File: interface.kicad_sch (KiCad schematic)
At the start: 8 parts

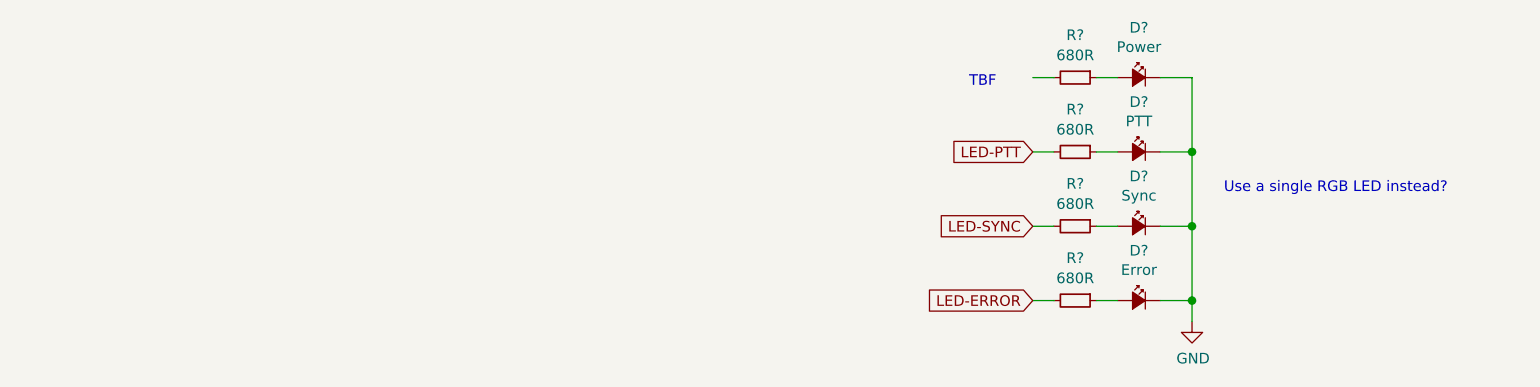
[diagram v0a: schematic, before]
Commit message: Add files via upload
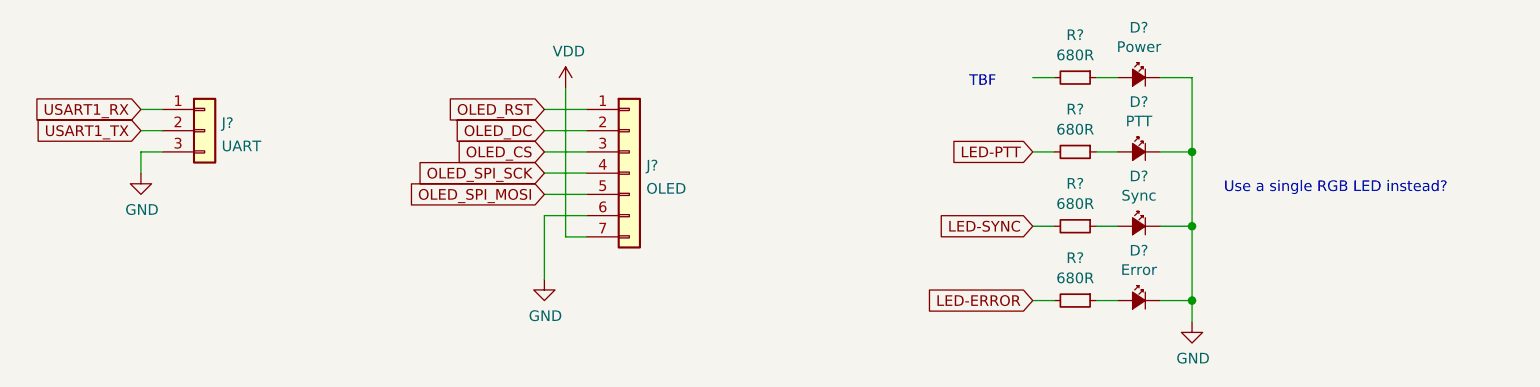
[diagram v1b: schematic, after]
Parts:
- added J?: OLED, Connector_PinHeader_2.54mm:PinHeader_1x07_P2.54mm_Vertical, symbol Connector_Generic:Conn_01x07
- added J?: UART, Connector_PinHeader_2.54mm:PinHeader_1x03_P2.54mm_Vertical, symbol Connector_Generic:Conn_01x03
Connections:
- net GND: now also J?.3 (Pin_3), J?.6 (Pin_6)
- new net OLED_CS: J?.3 (Pin_3)
- new net OLED_DC: J?.2 (Pin_2)
- new net OLED_RST: J?.1 (Pin_1)
- new net OLED_SPI_MOSI: J?.5 (Pin_5)
- new net OLED_SPI_SCK: J?.4 (Pin_4)
- new net USART1_RX: J?.1 (Pin_1)
- new net USART1_TX: J?.2 (Pin_2)
- new net VDD: J?.7 (Pin_7)
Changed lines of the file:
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@@
+    (stroke (width 0) (type solid) (color 0 0 0 0))
+  )
+  (wire (pts (xy 130.81 93.98) (xy 135.89 93.98))
     (stroke (width 0) (type solid) (color 0 0 0 0))
   )
@@
     (stroke (width 0) (type solid) (color 0 0 0 0))
   )
+  (wire (pts (xy 82.55 96.52) (xy 85.09 96.52))
+    (stroke (width 0) (type solid) (color 0 0 0 0))
+  )
   (wire (pts (xy 204.47 90.17) (xy 208.28 90.17))
     (stroke (width 0) (type solid) (color 0 0 0 0))
@@
     (stroke (width 0) (type solid) (color 0 0 0 0))
   )
+  (wire (pts (xy 135.89 106.68) (xy 130.81 106.68))
+    (stroke (width 0) (type solid) (color 0 0 0 0))
+  )
   (wire (pts (xy 208.28 116.84) (xy 208.28 119.38))
     (stroke (width 0) (type solid) (color 0 0 0 0))
@@
     (stroke (width 0) (type solid) (color 0 0 0 0))
   )
+  (wire (pts (xy 135.89 109.22) (xy 133.35 109.22))
+    (stroke (width 0) (type solid) (color 0 0 0 0))
+  )
   (wire (pts (xy 208.28 107.95) (xy 208.28 116.84))
     (stroke (width 0) (type solid) (color 0 0 0 0))
   )
+  (wire (pts (xy 133.35 109.22) (xy 133.35 91.44))
+    (stroke (width 0) (type solid) (color 0 0 0 0))
+  )
+  (wire (pts (xy 82.55 93.98) (xy 85.09 93.98))
+    (stroke (width 0) (type solid) (color 0 0 0 0))
+  )
   (wire (pts (xy 208.28 90.17) (xy 208.28 99.06))
     (stroke (width 0) (type solid) (color 0 0 0 0))
   )
+  (wire (pts (xy 130.81 101.6) (xy 135.89 101.6))
+    (stroke (width 0) (type solid) (color 0 0 0 0))
+  )
   (wire (pts (xy 196.85 99.06) (xy 199.39 99.06))
     (stroke (width 0) (type solid) (color 0 0 0 0))
   )
+  (wire (pts (xy 130.81 96.52) (xy 135.89 96.52))
+    (stroke (width 0) (type solid) (color 0 0 0 0))
+  )
+  (wire (pts (xy 130.81 106.68) (xy 130.81 114.3))
+    (stroke (width 0) (type solid) (color 0 0 0 0))
+  )
+  (wire (pts (xy 85.09 99.06) (xy 82.55 99.06))
+    (stroke (width 0) (type solid) (color 0 0 0 0))
+  )
   (wire (pts (xy 191.77 90.17) (xy 189.23 90.17))
     (stroke (width 0) (type solid) (color 0 0 0 0))
   )
   (wire (pts (xy 204.47 107.95) (xy 208.28 107.95))
+    (stroke (width 0) (type solid) (color 0 0 0 0))
+  )
+  (wire (pts (xy 82.55 99.06) (xy 82.55 101.6))
+    (stroke (width 0) (type solid) (color 0 0 0 0))
+  )
+  (wire (pts (xy 130.81 99.06) (xy 135.89 99.06))
+    (stroke (width 0) (type solid) (color 0 0 0 0))
+  )
+  (wire (pts (xy 130.81 104.14) (xy 135.89 104.14))
     (stroke (width 0) (type solid) (color 0 0 0 0))
   )
@@
     (effects (font (size 1.27 1.27)) (justify left bottom))
   )
+  (global_label "OLED_SPI_SCK" (shape input) (at 130.81 101.6 180) (fields_autoplaced)
+    (effects (font (size 1.27 1.27)) (justify right))
+    (property "Intersheet References" "${INTERSHEET_REFS}" (id 0) (at 114.9899 101.5206 0)
+      (effects (font (size 1.27 1.27)) (justify right) hide)
+    )
+  )
+  (global_label "OLED_DC" (shape input) (at 130.81 96.52 180) (fields_autoplaced)
+    (effects (font (size 1.27 1.27)) (justify right))
+    (property "Intersheet References" "${INTERSHEET_REFS}" (id 0) (at 120.2514 96.4406 0)
+      (effects (font (size 1.27 1.27)) (justify right) hide)
+    )
+  )
   (global_label "LED-PTT" (shape input) (at 189.23 99.06 180) (fields_autoplaced)
     (effects (font (size 1.27 1.27)) (justify right))
@@
     )
   )
+  (global_label "OLED_SPI_MOSI" (shape input) (at 130.81 104.14 180) (fields_autoplaced)
+    (effects (font (size 1.27 1.27)) (justify right))
+    (property "Intersheet References" "${INTERSHEET_REFS}" (id 0) (at 114.1433 104.0606 0)
+      (effects (font (size 1.27 1.27)) (justify right) hide)
+    )
+  )
   (global_label "LED-SYNC" (shape input) (at 189.23 107.95 180) (fields_autoplaced)
     (effects (font (size 1.27 1.27)) (justify right))
@@
     )
   )
+  (global_label "USART1_RX" (shape input) (at 82.55 93.98 180) (fields_autoplaced)
+    (effects (font (size 1.27 1.27)) (justify right))
+    (property "Intersheet References" "${INTERSHEET_REFS}" (id 0) (at 69.7537 94.0594 0)
+      (effects (font (size 1.27 1.27)) (justify right) hide)
+    )
+  )
+  (global_label "USART1_TX" (shape input) (at 82.55 96.52 180) (fields_autoplaced)
+    (effects (font (size 1.27 1.27)) (justify right))
+    (property "Intersheet References" "${INTERSHEET_REFS}" (id 0) (at 70.0561 96.5994 0)
+      (effects (font (size 1.27 1.27)) (justify right) hide)
+    )
+  )
+  (global_label "OLED_CS" (shape input) (at 130.81 99.06 180) (fields_autoplaced)
+    (effects (font (size 1.27 1.27)) (justify right))
+    (property "Intersheet References" "${INTERSHEET_REFS}" (id 0) (at 120.3118 98.9806 0)
+      (effects (font (size 1.27 1.27)) (justify right) hide)
+    )
+  )
   (global_label "LED-ERROR" (shape input) (at 189.23 116.84 180) (fields_autoplaced)
     (effects (font (size 1.27 1.27)) (justify right))
     (property "Intersheet References" "${INTERSHEET_REFS}" (id 0) (at -72.39 -38.1 0)
       (effects (font (size 1.27 1.27)) hide)
+    )
+  )
+  (global_label "OLED_RST" (shape input) (at 130.81 93.98 180) (fields_autoplaced)
+    (effects (font (size 1.27 1.27)) (justify right))
+    (property "Intersheet References" "${INTERSHEET_REFS}" (id 0) (at 119.3442 93.9006 0)
+      (effects (font (size 1.27 1.27)) (justify right) hide)
     )
   )
@@
     (pin "C")
   )
+  (symbol (lib_id "power:GND") (at 82.55 101.6 0) (unit 1)
+    (in_bom yes) (on_board yes)
+    (property "Reference" "#PWR?" (id 0) (at 82.55 107.95 0)
+      (effects (font (size 1.27 1.27)) hide)
+    )
+    (property "Value" "GND" (id 1) (at 82.677 105.9942 0))
+    (property "Footprint" "" (id 2) (at 82.55 101.6 0)
+      (effects (font (size 1.27 1.27)) hide)
+    )
+    (property "Datasheet" "" (id 3) (at 82.55 101.6 0)
+      (effects (font (size 1.27 1.27)) hide)
+    )
+    (pin "1")
+  )
+  (symbol (lib_id "power:VDD") (at 133.35 91.44 0) (unit 1)
+    (in_bom yes) (on_board yes)
+    (property "Reference" "#PWR?" (id 0) (at 133.35 95.25 0)
+      (effects (font (size 1.27 1.27)) hide)
+    )
+    (property "Value" "VDD" (id 1) (at 133.731 87.0458 0))
+    (property "Footprint" "" (id 2) (at 133.35 91.44 0)
+      (effects (font (size 1.27 1.27)) hide)
+    )
+    (property "Datasheet" "" (id 3) (at 133.35 91.44 0)
+      (effects (font (size 1.27 1.27)) hide)
+    )
+    (pin "1")
+  )
+  (symbol (lib_id "Connector_Generic:Conn_01x07") (at 140.97 101.6 0) (unit 1)
+    (in_bom yes) (on_board yes) (fields_autoplaced)
+    (property "Reference" "J?" (id 0) (at 143.0021 100.6915 0)
+      (effects (font (size 1.27 1.27)) (justify left))
+    )
+    (property "Value" "OLED" (id 1) (at 143.0021 103.4666 0)
+      (effects (font (size 1.27 1.27)) (justify left))
+    )
+    (property "Footprint" "Connector_PinHeader_2.54mm:PinHeader_1x07_P2.54mm_Vertical" (id 2) (at 140.97 101.6 0)
+      (effects (font (size 1.27 1.27)) hide)
+    )
+    (property "Datasheet" "~" (id 3) (at 140.97 101.6 0)
+      (effects (font (size 1.27 1.27)) hide)
+    )
+    (pin "1")
+    (pin "2")
+    (pin "3")
+    (pin "4")
+    (pin "5")
+    (pin "6")
+    (pin "7")
+  )
   (symbol (lib_id "pkl_device:pkl_R_Small") (at 194.31 107.95 270) (unit 1)
     (in_bom yes) (on_board yes)
@@
     (pin "2")
   )
+  (symbol (lib_id "power:GND") (at 130.81 114.3 0) (unit 1)
+    (in_bom yes) (on_board yes)
+    (property "Reference" "#PWR?" (id 0) (at 130.81 120.65 0)
+      (effects (font (size 1.27 1.27)) hide)
+    )
+    (property "Value" "GND" (id 1) (at 130.937 118.6942 0))
+    (property "Footprint" "" (id 2) (at 130.81 114.3 0)
+      (effects (font (size 1.27 1.27)) hide)
+    )
+    (property "Datasheet" "" (id 3) (at 130.81 114.3 0)
+      (effects (font (size 1.27 1.27)) hide)
+    )
+    (pin "1")
+  )
   (symbol (lib_id "power:GND") (at 208.28 119.38 0) (unit 1)
     (in_bom yes) (on_board yes)
@@
     (pin "1")
   )
+  (symbol (lib_id "Connector_Generic:Conn_01x03") (at 90.17 96.52 0) (unit 1)
+    (in_bom yes) (on_board yes) (fields_autoplaced)
+    (property "Reference" "J?" (id 0) (at 92.2021 95.6115 0)
+      (effects (font (size 1.27 1.27)) (justify left))
+    )
+    (property "Value" "UART" (id 1) (at 92.2021 98.3866 0)
+      (effects (font (size 1.27 1.27)) (justify left))
+    )
+    (property "Footprint" "Connector_PinHeader_2.54mm:PinHeader_1x03_P2.54mm_Vertical" (id 2) (at 90.17 96.52 0)
+      (effects (font (size 1.27 1.27)) hide)
+    )
+    (property "Datasheet" "~" (id 3) (at 90.17 96.52 0)
+      (effects (font (size 1.27 1.27)) hide)
+    )
+    (pin "1")
+    (pin "2")
+    (pin "3")
+  )
 )
